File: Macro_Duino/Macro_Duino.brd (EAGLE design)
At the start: 68.6 x 53.3 mm, 21 parts, among them J2 KLDX-0202-A, U1 ATMEGA328P-AU, X1 ABMM-16.000MHZ-B2-T

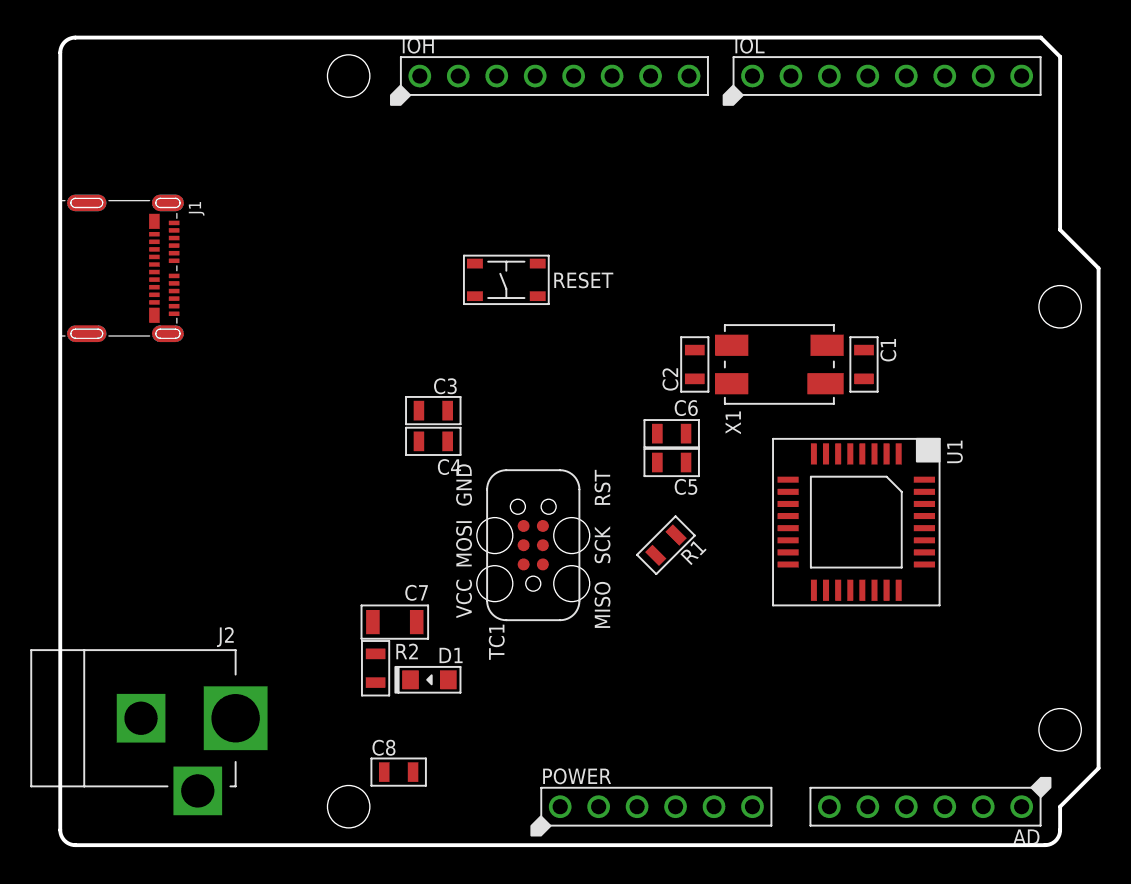
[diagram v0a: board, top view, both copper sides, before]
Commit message: Almost done with Macro Duino
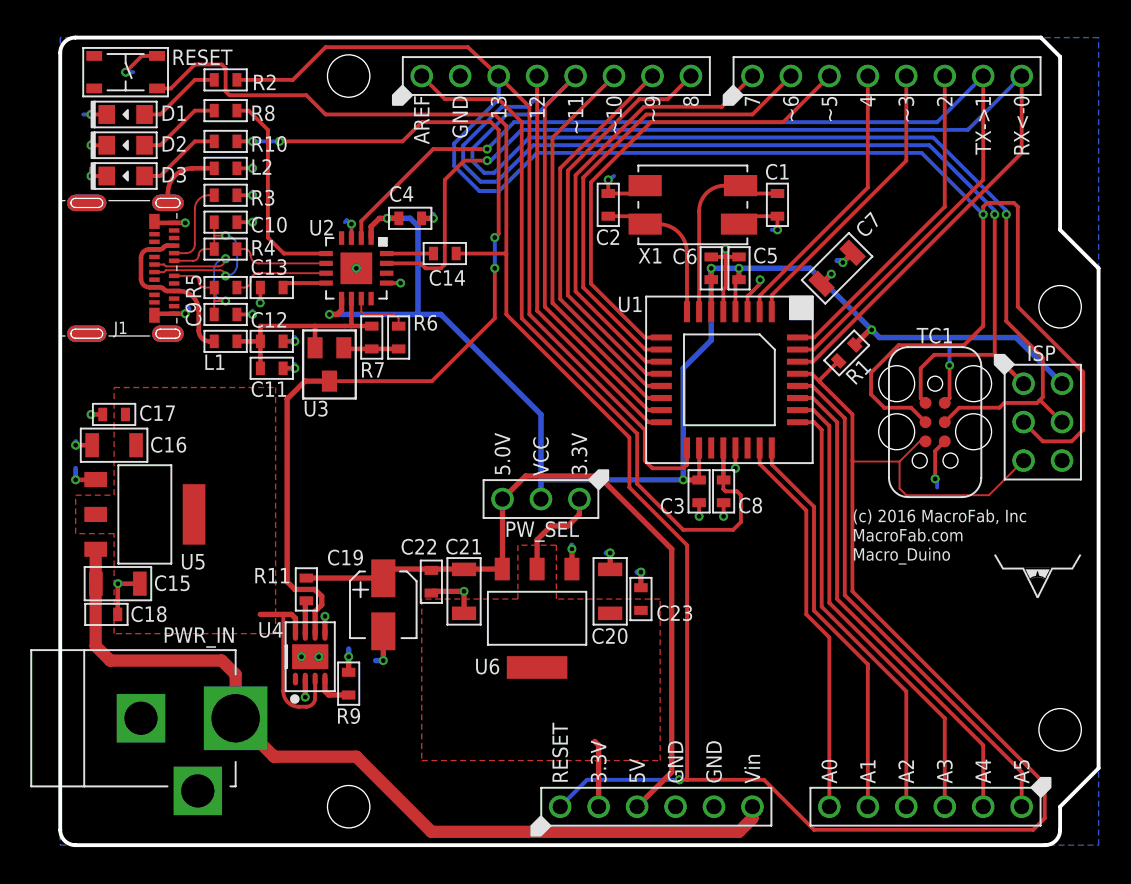
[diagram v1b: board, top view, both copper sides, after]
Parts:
- added C10, C9: 47pF, MF_Passives:C0603
- added C11, C13, C14, C17, C18, C22, C23: 0.1uF, MF_Passives:C0603
- added C12: 1uF, MF_Passives:C0603
- added C15, C16, C20, C21: 10uF, MF_Passives:C1206
- added C19: MF-CAP-4MM-10uF, MF_Passives:CP4MM
- added D2, D3: MF-LED-0805-RED, MF_LEDs:LED0805
- added FRAME1: MF_FRAMEDEFAULT, MF_Aesthetics:MF_FRAME_DEFAULT
- added ISP: MF-CON-2.54mm-2x3, MF_Connectors:PTH_2.54MM_02X03
- added L1, L2: MI0603K300R-10, MF_Passives:L0603
- added PW_SEL: MF-CON-2.54mm-01x03, MF_Connectors:PTH_2.54MM_01X03
- added R10, R8: 360, MF_Passives:R0603
- added R11: 0, MF_Passives:R0603
- added R3: 5.1K, MF_Passives:R0603
- added R4, R5: 27, MF_Passives:R0603
- added R6, R9: 1K, MF_Passives:R0603
- added R7: 100K, MF_Passives:R0603
- added U$14: MF_LOGOLOGO_TEXT, PP_Aesthetics:MF_LOGO_TEXT
- added U$15: LHE_LOGOLHE_LOGO, PP_Aesthetics:LHE_LOGO
- added U2: FT230XQ-R, PP_DigitalIC:FT230X_QFN-16
- added U3: (no value), PP_DiscreteSemi:SOT-23-3
- added U4: TPS2113ADRBR, PP_PowerIC:TPS211X_SON-8
- added U5: NCP1117LPST50T3G, MF_IC_Power:SOT-223-3
- added U6: NCP1117LPST33T3G, MF_IC_Power:SOT-223-3
- C1, C2, C3, C4, C5, C6, C8: device MF_Passives:C0805 -> MF_Passives:C0603
- J1: value (none) -> 105450-0101
- R1, R2: device MF_Passives:R0805 -> MF_Passives:R0603
- U1: value ATMEGA328P-AU -> ATMEGA328PB-AU
- moved D1 42.4 mm to (4.32, 48.3)
- moved R2 40.1 mm to (10.9, 50.5), turned to 180 degrees
- moved C7 37.4 mm to (51.3, 38.1), turned to 45 degrees
- moved RESET 28.6 mm to (4.32, 51.1), turned to 180 degrees
- moved C8 28.4 mm to (43.8, 23.4), turned to 270 degrees
- moved TC1 27.8 mm to (57.8, 27.9), turned to 270 degrees
- moved C3 18.4 mm to (42.2, 23.4), turned to 270 degrees
- moved R1 17.4 mm to (51.9, 32.5)
- moved C4 14.8 mm to (23.1, 41.4), turned to 0 degrees
- moved C5 13.6 mm to (44.8, 38.1), turned to 90 degrees
- moved U1 12.6 mm to (44.2, 30.7)
- moved C1 12.0 mm to (47.4, 42.3)
- moved C2 12.0 mm to (36.2, 42.3)
- moved X1 12.0 mm to (41.8, 42.3)
- moved C6 11.2 mm to (43.0, 38.1), turned to 90 degrees
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- renumbered J2 to PWR_IN
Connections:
- removed net PD0: IOL.P$8, U1.P$30
- removed net PD1: IOL.P$7, U1.P$31
- removed net PIN: PWR_IN.PIN
- removed net SLEEVE: PWR_IN.SLEEVE1
- removed net SLEEVE_SHUNT: PWR_IN.SLEEVE2
- new net 3V3OUT: C13.P$1, U2.8
- new net CC1: J1.A5, R3.P$1
- new net D+: R4.P$2, U2.6
- new net D-: R5.P$2, U2.7
- new net ILIM: R9.P$1, U4.4
- new net N$1: D3.ANODE, R10.P$1
- new net N$3: R11.P$1, U4.7
- new net PW_EN: R6.P$2, U2.11
- new net PW_GT: R6.P$1, R7.P$1, U3.1
- new net RTS: C14.P$2, U2.16
- new net RXD: IOL.P$7, U1.P$31, U2.2
- new net TXD: IOL.P$8, U1.P$30, U2.15
- new net TX_RX_LED: R8.P$1, U2.5
- new net TX_RX_LED_1: D2.ANODE, R8.P$2
- new net USB_5.0V_0: J1.A4, J1.A9, J1.B4, J1.B9, L1.P$1
- new net USB_5.0V_1: C11.P$1, C12.P$1, L1.P$2, R7.P$2, U2.10, U3.2
- new net USB_D+: C10.P$1, J1.A6, J1.B6, R4.P$1
- new net USB_D-: C9.P$1, J1.A7, J1.B7, R5.P$1
- new net USB_SHLD: J1.S_T1, J1.S_T2, J1.S_T3, J1.S_T4, L2.P$1
- new net USB_SW_5.0V: R10.P$2, U3.3, U4.6
- new net VCC: C3.P$1, C4.P$1, C5.P$1, C6.P$1, C7.P$1, ISP.P$2, PW_SEL.P$2, R1.P$1, TC1.P$2, U1.P$18, U1.P$4, U1.P$6, U2.1, U2.9
- new net VIN_5.0V: C16.P$1, C17.P$1, U4.3, U4.8, U5.P$1, U5.P$3
- net 3.3V: now also C20.P$1, C23.P$1, PW_SEL.P$1, U6.P$1, U6.P$3
- net 5.0V: now also C19.P$1, C21.P$1, C22.P$1, PW_SEL.P$3, R11.P$2, U6.P$4; no longer C3.P$1, C4.P$1, C5.P$1, C6.P$1, C7.P$1, R1.P$1, TC1.P$2, U1.P$18, U1.P$4, U1.P$6
- net GND: now also C10.P$2, C11.P$2, C12.P$2, C13.P$2, C15.P$2, C16.P$2, C17.P$2, C18.P$2, C19.P$2, C20.P$2, C21.P$2, C22.P$2, C23.P$2, C9.P$2, D1.CATHODE, D2.CATHODE, D3.CATHODE, ISP.P$6, J1.A1, J1.A12, J1.B1, J1.B12, L2.P$2, PWR_IN.SLEEVE1, PWR_IN.SLEEVE2, R3.P$2, R9.P$2, U2.13, U2.3, U2.PAD, U4.2, U4.5, U4.PAD, U5.P$2, U6.P$2; no longer R2.P$2
- net MISO: now also ISP.P$1
- net MOSI: now also ISP.P$4
- net N$2: now also D1.ANODE, R2.P$2; no longer D1.CATHODE, R2.P$1
- net RST: now also C14.P$1, ISP.P$5
- net SCK: now also ISP.P$3, R2.P$1; no longer D1.ANODE
- net VIN: now also C15.P$1, C18.P$1, PWR_IN.PIN, U5.P$4
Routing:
- net RST: track 0.00 -> 167.2 mm, vias 0 -> 1
- net SCK: track 0.00 -> 144.2 mm, vias 0 -> 1
- net VCC: track 0.00 -> 102.0 mm, vias 0 -> 8
- net MOSI: track 0.00 -> 97.3 mm, vias 0 -> 1
- net MISO: track 0.00 -> 96.4 mm, vias 0 -> 1
- net TXD: track 0.00 -> 76.2 mm, vias 0 -> 1
- net GND: track 0.00 -> 71.8 mm, vias 0 -> 40
- net RXD: track 0.00 -> 69.9 mm, vias 0 -> 1
- net USB_SW_5.0V: track 0.00 -> 63.9 mm, vias 0 -> 4
- net VIN: track 0.00 -> 60.0 mm
- net AREF: track 0.00 -> 51.2 mm
- net 5.0V: track 0.00 -> 50.0 mm
- net PC5: track 0.00 -> 34.5 mm
- net PC4: track 0.00 -> 32.7 mm
- net PD5: track 0.00 -> 31.5 mm
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- added copper zone on layer 1, net 3.3V
- added copper zone on layer 16, net GND
- added copper zone on layer 1, net VIN_5.0V

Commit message: Complete!~
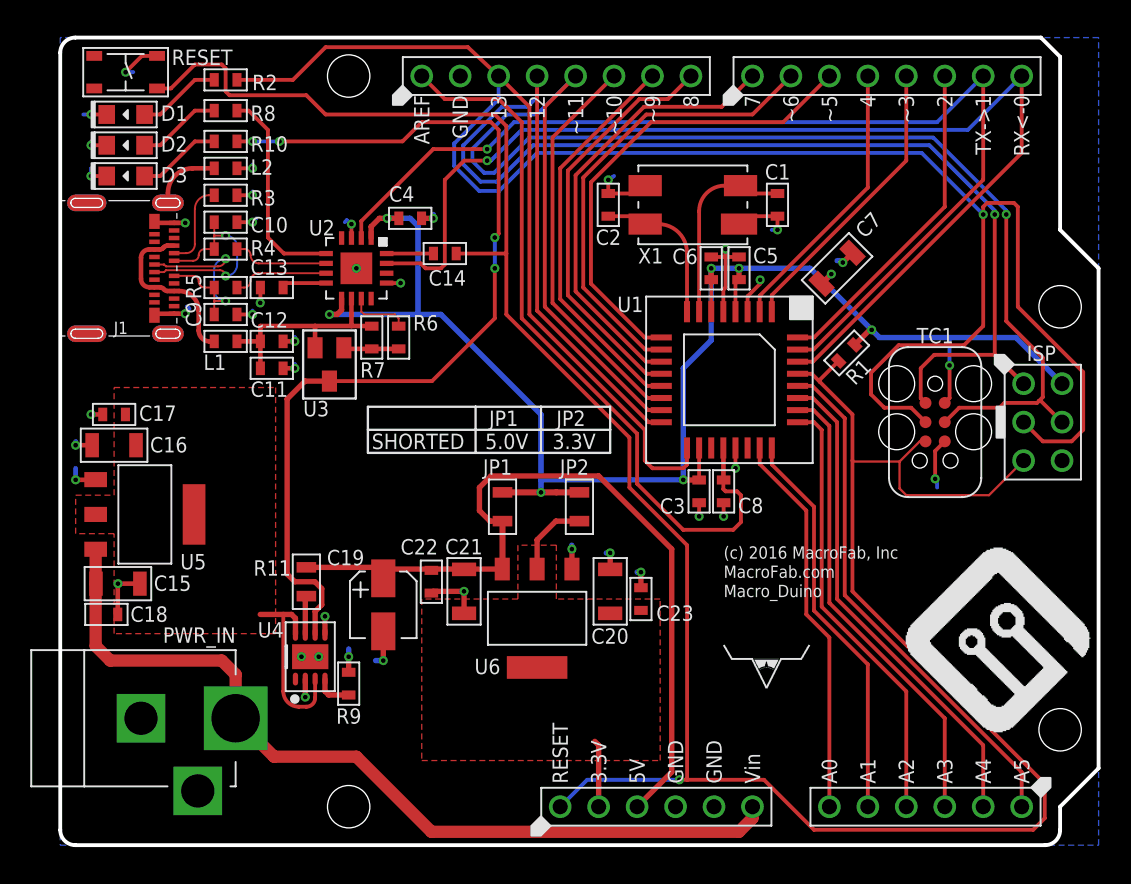
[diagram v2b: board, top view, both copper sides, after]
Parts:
- removed PW_SEL: MF-CON-2.54mm-01x03, MF_Connectors:PTH_2.54MM_01X03
- added JP1, JP2: 0, MF_Passives:R0805
- R11: device MF_Passives:R0603 -> MF_Passives:R0805
- U$14: value MF_LOGOLOGO_TEXT -> MF_LOGOLOGO; device PP_Aesthetics:MF_LOGO_TEXT -> PP_Aesthetics:MF_LOGO
- U3: value (none) -> IRLML6401TRPBF
- moved U$15 18.9 mm to (48.6, 10.3)
- moved U$14 10.2 mm to (55.9, 7.49), flipped to the top
- moved FRAME1 8.84 mm to (43.8, 20.2)
- moved R11 0.51 mm to (16.3, 17.4)
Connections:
- net 3.3V: now also JP2.P$1; no longer PW_SEL.P$1
- net 5.0V: now also JP1.P$2; no longer PW_SEL.P$3
- net VCC: now also JP1.P$1, JP2.P$2; no longer PW_SEL.P$2
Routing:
- net VCC: track 102.0 -> 106.7 mm, vias 8 -> 9
- net 5.0V: track 50.0 -> 53.8 mm
- net 3.3V: track 10.9 -> 9.66 mm
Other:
- board text added: "3.3V"
- board text added: "5.0V"
- board text added: "C:/Users/Parker/Desktop/MacroDuino_Back_silkscreen.bmp"
- board text added: "JP1"
- board text added: "JP2"
- board text added: "SHORTED"
